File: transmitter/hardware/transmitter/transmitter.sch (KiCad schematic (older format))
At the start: 26 parts, among them J1 SOIL, J2 SOIL, J3 USB_UART, J4 PWR, J5 SOIL, J6 SOIL, J7 SOIL, J8 SOIL, SW1 SW_SPST, SW2 SW, U1 NodeMCU_1.0_(ESP-12E), U2 MCP1700-3302E_SOT89, U3 CD4051B

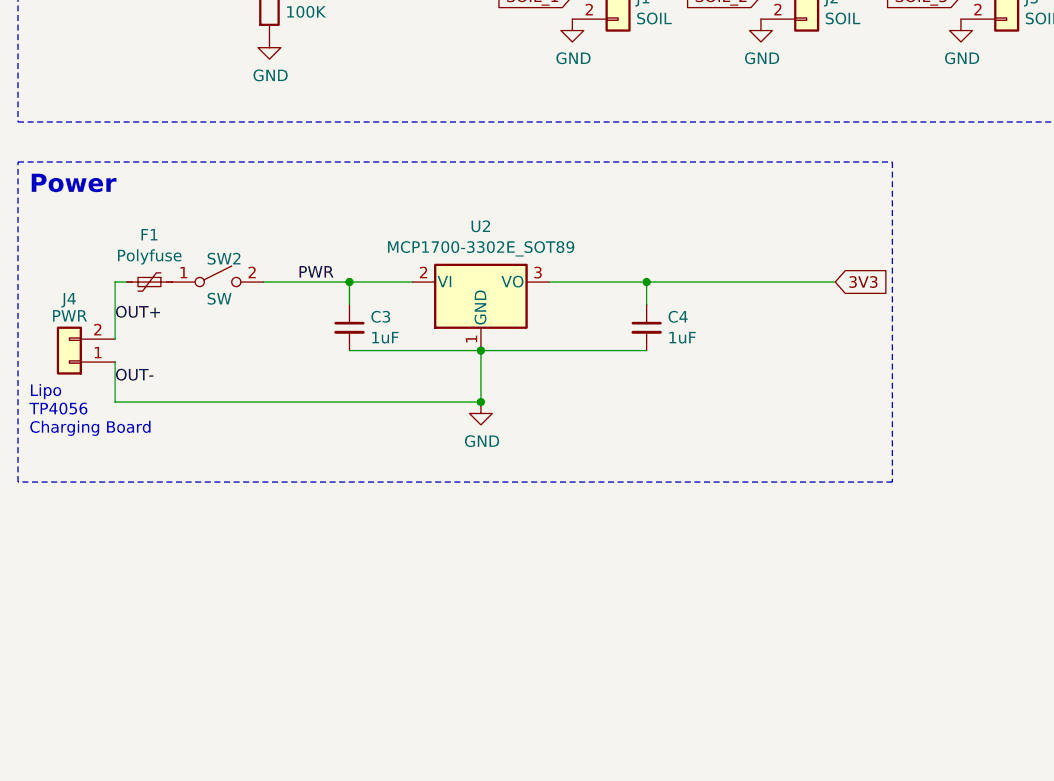
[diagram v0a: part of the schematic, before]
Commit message: Alternate LDO
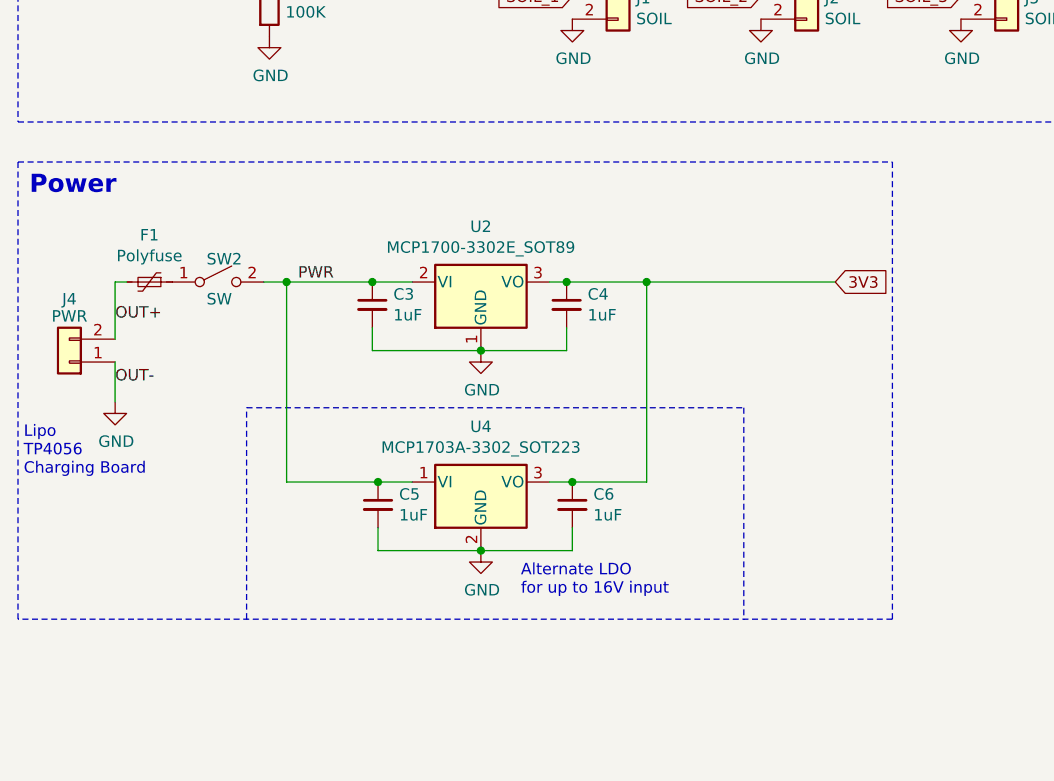
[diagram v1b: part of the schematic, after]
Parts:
- added C5, C6: 1uF, Capacitor_SMD:C_0603_1608Metric_Pad1.05x0.95mm_HandSolder, symbol Device:C_Small
- added U4: MCP1703A-3302_SOT223, Package_TO_SOT_SMD:SOT-223-3_TabPin2, symbol Regulator_Linear:MCP1703A-3302_SOT223
- J4: footprint Connector_PinHeader_2.54mm:PinHeader_1x02_P2.54mm_Vertical -> tp4056:tp4056
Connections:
- net 3V3: now also C6.1, U4.3 (VO)
- net GND: now also C5.2, C6.2, U4.2 (GND)
- net PWR: now also C5.1, U4.1 (VI)
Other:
- note added: "Alternate LDO\nfor up to 16V input"
- moved on the sheet: C3, C4
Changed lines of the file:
@@
 L power:GND #PWR06
 U 1 1 5DBC1A3A
-P 2625 3125
-F 0 "#PWR06" H 2625 2875 50  0001 C CNN
-F 1 "GND" H 2630 2952 50  0000 C CNN
-F 2 "" H 2625 3125 50  0001 C CNN
-F 3 "" H 2625 3125 50  0001 C CNN
-	1    2625 3125
+P 2625 2900
+F 0 "#PWR06" H 2625 2650 50  0001 C CNN
+F 1 "GND" H 2630 2727 50  0000 C CNN
+F 2 "" H 2625 2900 50  0001 C CNN
+F 3 "" H 2625 2900 50  0001 C CNN
+	1    2625 2900
 	1    0    0    -1
 $EndComp
@@
 L Device:C_Small C3
 U 1 1 5DBC2404
-P 2050 2800
-F 0 "C3" H 2142 2846 50  0000 L CNN
-F 1 "1uF" H 2142 2755 50  0000 L CNN
-F 2 "Capacitor_SMD:C_0603_1608Metric_Pad1.05x0.95mm_HandSolder" H 2050 2800 50  0001 C CNN
-F 3 "~" H 2050 2800 50  0001 C CNN
-	1    2050 2800
+P 2150 2700
+F 0 "C3" H 2242 2746 50  0000 L CNN
+F 1 "1uF" H 2242 2655 50  0000 L CNN
+F 2 "Capacitor_SMD:C_0603_1608Metric_Pad1.05x0.95mm_HandSolder" H 2150 2700 50  0001 C CNN
+F 3 "~" H 2150 2700 50  0001 C CNN
+	1    2150 2700
 	1    0    0    -1
 $EndComp
@@
 L Device:C_Small C4
 U 1 1 5DBC2493
-P 3350 2800
-F 0 "C4" H 3442 2846 50  0000 L CNN
-F 1 "1uF" H 3442 2755 50  0000 L CNN
-F 2 "Capacitor_SMD:C_0603_1608Metric_Pad1.05x0.95mm_HandSolder" H 3350 2800 50  0001 C CNN
-F 3 "~" H 3350 2800 50  0001 C CNN
-	1    3350 2800
+P 3000 2700
+F 0 "C4" H 3092 2746 50  0000 L CNN
+F 1 "1uF" H 3092 2655 50  0000 L CNN
+F 2 "Capacitor_SMD:C_0603_1608Metric_Pad1.05x0.95mm_HandSolder" H 3000 2700 50  0001 C CNN
+F 3 "~" H 3000 2700 50  0001 C CNN
+	1    3000 2700
 	1    0    0    -1
 $EndComp
-Wire Wire Line
-	3350 2700 3350 2600
-Wire Wire Line
-	3350 2600 2925 2600
-Wire Wire Line
-	2050 2700 2050 2600
-Wire Wire Line
-	2050 2900 2625 2900
-Wire Wire Line
-	3350 2900 2625 2900
-Connection ~ 2625 2900
 Text Label 1825 2600 0    50   ~ 0
 PWR
@@
 Text GLabel 4175 2600 2    50   Input ~ 0
 3V3
-Wire Wire Line
-	3350 2600 4175 2600
-Connection ~ 3350 2600
 Text GLabel 6025 4325 0    50   Input ~ 0
 3V3
@@
 	600  2075 4425 2075
 Wire Notes Line
-	4425 2075 4425 3475
-Wire Notes Line
-	4425 3475 600  3475
-Wire Notes Line
-	600  3475 600  2075
+	4425 4075 600  4075
 Text Notes 650  2225 0    79   ~ 16
 Power
@@
 	1    0    0    -1
 $EndComp
-Wire Wire Line
-	1675 2600 2050 2600
-Wire Wire Line
-	2050 2600 2325 2600
-Connection ~ 2050 2600
 $Comp
 L Connector_Generic:Conn_01x02 J3
@@
 F 0 "J4" H 825 2675 50  0000 C CNN
 F 1 "PWR" H 825 2750 50  0000 C CNN
-F 2 "Connector_PinHeader_2.54mm:PinHeader_1x02_P2.54mm_Vertical" H 825 2950 50  0001 C CNN
+F 2 "tp4056:tp4056" H 825 2950 50  0001 C CNN
 F 3 "~" H 825 2950 50  0001 C CNN
 	1    825  2950
 	-1   0    0    1
 $EndComp
-Wire Wire Line
-	2625 2900 2625 3125
-Text Notes 650  3275 0    50   ~ 0
+Text Notes 625  3450 0    50   ~ 0
 Lipo \nTP4056\nCharging Board
 Wire Wire Line
@@
 Wire Wire Line
 	1025 2950 1025 3125
-Wire Wire Line
-	1025 3125 2625 3125
-Connection ~ 2625 3125
 Text Label 1025 2775 0    50   ~ 0
 OUT+
 Text Label 1025 3050 0    50   ~ 0
 OUT-
+$Comp
+L Regulator_Linear:MCP1703A-3302_SOT223 U4
+U 1 1 5DC182DA
+P 2625 3475
+F 0 "U4" H 2625 3717 50  0000 C CNN
+F 1 "MCP1703A-3302_SOT223" H 2625 3626 50  0000 C CNN
+F 2 "Package_TO_SOT_SMD:SOT-223-3_TabPin2" H 2625 3675 50  0001 C CNN
+F 3 "http://ww1.microchip.com/downloads/en/DeviceDoc/20005122B.pdf" H 2625 3425 50  0001 C CNN
+	1    2625 3475
+	1    0    0    -1
+$EndComp
+Wire Wire Line
+	2325 3475 2175 3475
+Wire Wire Line
+	2925 3475 3025 3475
+$Comp
+L power:GND #PWR016
+U 1 1 5DC1D21C
+P 2625 3775
+F 0 "#PWR016" H 2625 3525 50  0001 C CNN
+F 1 "GND" H 2630 3602 50  0000 C CNN
+F 2 "" H 2625 3775 50  0001 C CNN
+F 3 "" H 2625 3775 50  0001 C CNN
+	1    2625 3775
+	1    0    0    -1
+$EndComp
+$Comp
+L power:GND #PWR015
+U 1 1 5DC1E5D1
+P 1025 3125
+F 0 "#PWR015" H 1025 2875 50  0001 C CNN
+F 1 "GND" H 1030 2952 50  0000 C CNN
+F 2 "" H 1025 3125 50  0001 C CNN
+F 3 "" H 1025 3125 50  0001 C CNN
+	1    1025 3125
+	1    0    0    -1
+$EndComp
+Wire Notes Line
+	600  2075 600  4075
+Wire Notes Line
+	4425 2075 4425 4075
+Connection ~ 3000 2600
+Wire Wire Line
+	3000 2600 2925 2600
+Connection ~ 2150 2600
+Wire Wire Line
+	2150 2600 2325 2600
+Wire Wire Line
+	1675 2600 1775 2600
+Wire Wire Line
+	3000 2600 3350 2600
+Wire Wire Line
+	2150 2800 2150 2900
+Wire Wire Line
+	2150 2900 2625 2900
+Connection ~ 2625 2900
+Wire Wire Line
+	2625 2900 3000 2900
+Wire Wire Line
+	3000 2900 3000 2800
+$Comp
+L Device:C_Small C5
+U 1 1 5DC24C67
+P 2175 3575
+F 0 "C5" H 2267 3621 50  0000 L CNN
+F 1 "1uF" H 2267 3530 50  0000 L CNN
+F 2 "Capacitor_SMD:C_0603_1608Metric_Pad1.05x0.95mm_HandSolder" H 2175 3575 50  0001 C CNN
+F 3 "~" H 2175 3575 50  0001 C CNN
+	1    2175 3575
+	1    0    0    -1
+$EndComp
+Connection ~ 2175 3475
+$Comp
+L Device:C_Small C6
+U 1 1 5DC24CF9
+P 3025 3575
+F 0 "C6" H 3117 3621 50  0000 L CNN
+F 1 "1uF" H 3117 3530 50  0000 L CNN
+F 2 "Capacitor_SMD:C_0603_1608Metric_Pad1.05x0.95mm_HandSolder" H 3025 3575 50  0001 C CNN
+F 3 "~" H 3025 3575 50  0001 C CNN
+	1    3025 3575
+	1    0    0    -1
+$EndComp
+Connection ~ 3025 3475
+Wire Wire Line
+	3025 3475 3350 3475
+Wire Wire Line
+	2175 3675 2175 3775
+Wire Wire Line
+	2175 3775 2625 3775
+Connection ~ 2625 3775
+Wire Wire Line
+	2625 3775 3025 3775
+Wire Wire Line
+	3025 3775 3025 3675
+Wire Wire Line
+	1775 3475 1775 2600
+Wire Wire Line
+	1775 3475 2175 3475
+Connection ~ 1775 2600
+Wire Wire Line
+	1775 2600 2150 2600
+Wire Wire Line
+	3350 3475 3350 2600
+Connection ~ 3350 2600
+Wire Wire Line
+	3350 2600 4175 2600
+Text Notes 2800 3975 0    50   ~ 0
+Alternate LDO\nfor up to 16V input
+Wire Notes Line
+	1600 4075 1600 3150
+Wire Notes Line
+	1600 3150 3775 3150
+Wire Notes Line
+	3775 3150 3775 4075
 $EndSCHEMATC
